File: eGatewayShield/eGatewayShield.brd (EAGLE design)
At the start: 61.1 x 54.9 mm, 17 parts, among them SW1 SPST_TACT-EVQQ2, U1 ATMEGA328P_TQFP, U2 RFM69HW, X1 RASPI_BOARD_B+#_F, Y1 16MHZ

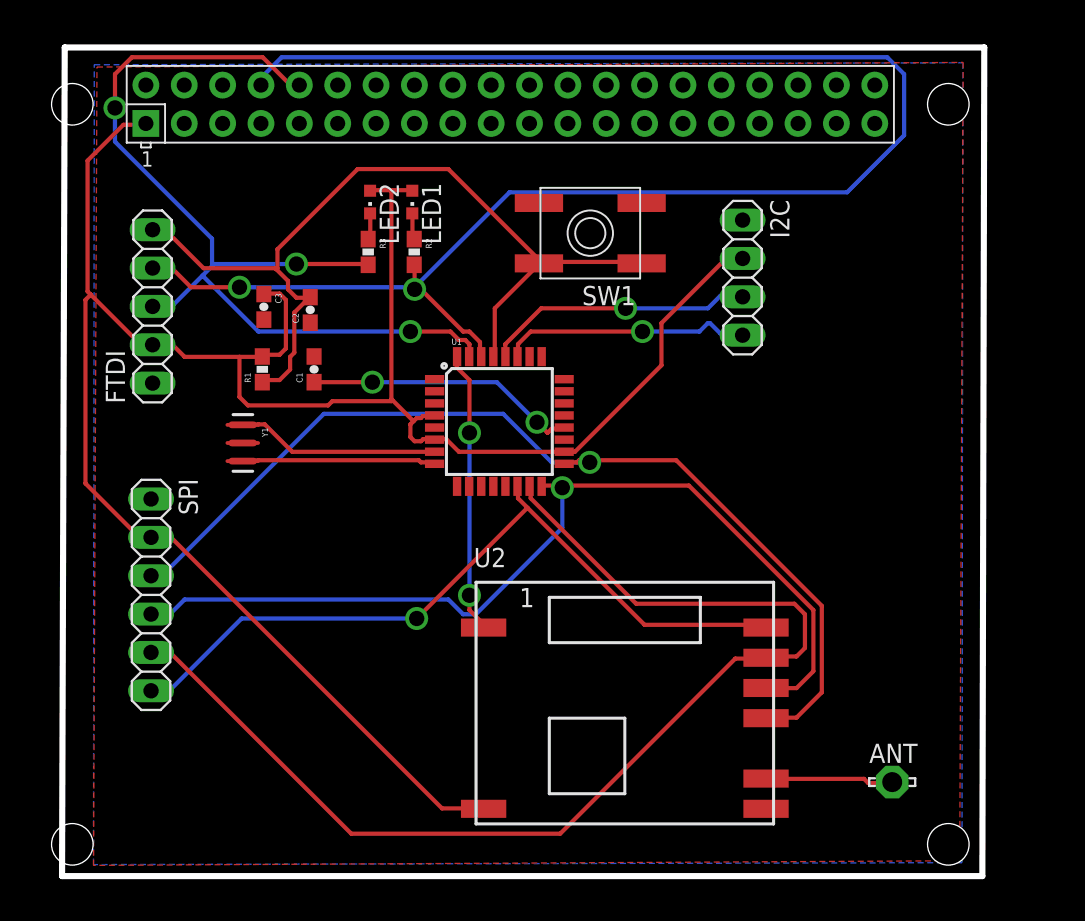
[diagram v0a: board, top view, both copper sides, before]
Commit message: Add Backup files from old smart home project
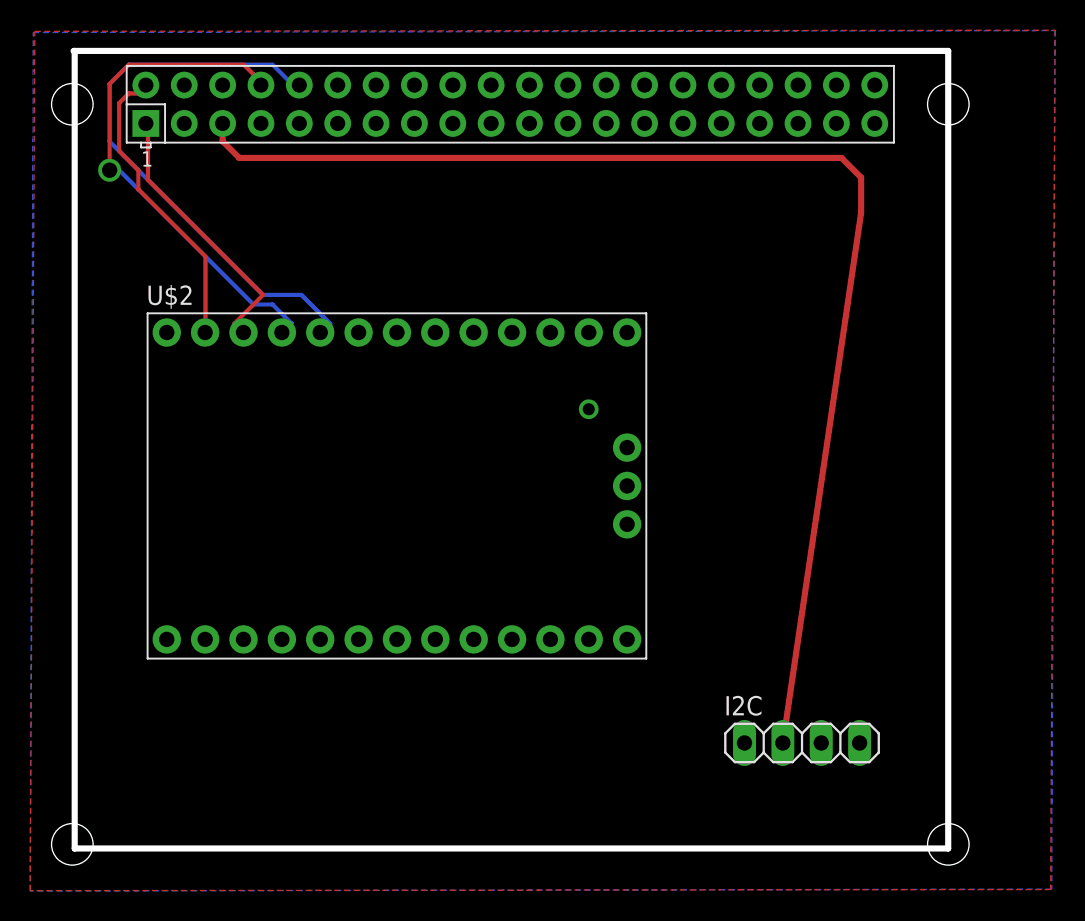
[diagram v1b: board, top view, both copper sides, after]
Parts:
- removed ANT: LSP13, solpad:LSP13
- removed C1, C2, C3: 0.1uF, SparkFun-Capacitors:0603-CAP
- removed FTDI: (no value), pinhead:1X05
- removed LED1, LED2: (no value), adafruit:CHIPLED_0603
- removed R1: (no value), SparkFun-Resistors:0603-RES
- removed R2, R3: 1K, SparkFun-Resistors:0603-RES
- removed SPI: (no value), pinhead:1X06
- removed SW1: SPST_TACT-EVQQ2, adafruit:EVQ-Q2
- removed U1: ATMEGA328P_TQFP, SparkFun-DigitalIC:TQFP32-08
- removed U2: RFM69HW, SparkFun-RF:RFM69W-XXXS2
- removed Y1: 16MHZ, SparkFun-FreqCtrl:RESONATOR-SMD
- added U$2: MOTEINO_R4_MODULEUSING_SQ_POST_PINS, MoteinoR4Mod:MOTEINTO_R4_SQ
- moved I2C 31.1 mm to (52.2, 10.3), turned to 0 degrees
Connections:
- removed net 5V0A: X1.2
- removed net A4/SDA: I2C.4, U1.27
- removed net A5/SCL: I2C.3, U1.28
- removed net ANT: ANT.MP, U2.10
- removed net D10/SS: SPI.6, U1.14, U2.15
- removed net D11/MOSI: SPI.5, U1.15, U2.14
- removed net D12/MISO: SPI.4, U1.16, U2.13
- removed net D13/SCK: SPI.3, U1.17, U2.12
- removed net D2: U1.32, U2.2
- removed net D3: U1.1
- removed net DTR: C2.1
- removed net N$1: LED1.C, R2.1
- removed net N$2: LED2.C, R3.1
- removed net N$7: C1.1, U1.20
- removed net RESET: C2.2, FTDI.5, R1.1, SW1.B, SW1.B', U1.29
- removed net RX: FTDI.4, R2.2, U1.30, X1.8
- removed net TX: FTDI.3, R3.2, U1.31, X1.10
- removed net XTAL1: U1.7, Y1.1
- removed net XTAL2: U1.8, Y1.3
- new net 5V: U$2.PWR, X1.2
- new net RXI: U$2.D1, X1.8
- new net SCL: I2C.2, X1.5
- new net SDA: I2C.1, X1.3
- new net TXO: U$2.D0, X1.10
- net 3.3V: now also I2C.4, U$2.3.3V; no longer C3.1, FTDI.2, I2C.2, LED1.A, LED2.A, R1.2, SPI.2, U1.18, U1.4, U1.6, U2.8
- net GND: now also I2C.3, U$2.G2, U$2.GND; no longer C1.2, C3.2, FTDI.1, I2C.1, SPI.1, SW1.A, SW1.A', U1.21, U1.3, U1.5, U2.9, Y1.2
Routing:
- net 3.3V: track 145.6 -> 18.1 mm
- net RX: track 111.3 -> 0.00 mm, vias 2 -> 0
- net SCL: track 0.00 -> 82.3 mm
- net D11/MOSI: track 77.8 -> 0.00 mm
- net D13/SCK: track 66.3 -> 0.00 mm, vias 1 -> 0
- net TX: track 64.6 -> 0.00 mm, vias 3 -> 0
- net D12/MISO: track 62.3 -> 0.00 mm, vias 1 -> 0
- net RESET: track 58.2 -> 0.00 mm
- net D10/SS: track 50.7 -> 0.00 mm, vias 1 -> 0
- net TXO: track 0.00 -> 38.4 mm
- net RXI: track 0.00 -> 34.8 mm, vias 0 -> 1
- net 5V: track 0.00 -> 19.8 mm
- net D2: track 18.7 -> 0.00 mm, vias 2 -> 0
- net N$7: track 18.1 -> 0.00 mm, vias 2 -> 0
- net A5/SCL: track 17.9 -> 0.00 mm, vias 1 -> 0
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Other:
- board size 61.1 x 54.9 mm -> 57.9 x 52.8 mm
